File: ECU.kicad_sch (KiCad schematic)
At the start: 0 parts

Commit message: ECU
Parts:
- added K1: Relay_DPDT, symbol Relay:Relay_DPDT
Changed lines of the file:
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@@
 	(generator_version "9.0")
 	(paper "A4")
+	(symbol
+		(lib_id "Relay:Relay_DPDT")
+		(at 140.97 80.01 270)
+		(unit 1)
+		(exclude_from_sim no)
+		(in_bom yes)
+		(on_board yes)
+		(dnp no)
+		(fields_autoplaced yes)
+		(property "Reference" "K1"
+			(at 140.97 59.69 90)
+			(effects
+				(font
+					(size 1.27 1.27)
+				)
+			)
+		)
+		(property "Value" "Relay_DPDT"
+			(at 140.97 62.23 90)
+			(effects
+				(font
+					(size 1.27 1.27)
+				)
+			)
+		)
+		(property "Footprint" ""
+			(at 139.7 96.52 0)
+			(effects
+				(font
+					(size 1.27 1.27)
+				)
+				(justify left)
+				(hide yes)
+			)
+		)
+		(property "Datasheet" "~"
+			(at 140.97 80.01 0)
+			(effects
+				(font
+					(size 1.27 1.27)
+				)
+				(hide yes)
+			)
+		)
+		(property "Description" "Relay DPDT, monostable, EN50005"
+			(at 140.97 80.01 0)
+			(effects
+				(font
+					(size 1.27 1.27)
+				)
+				(hide yes)
+			)
+		)
+		(pin "11"
+		)
+		(pin "22"
+		)
+		(pin "A1"
+		)
+		(pin "A2"
+		)
+		(pin "12"
+		)
+		(pin "14"
+		)
+		(pin "24"
+		)
+		(pin "21"
+		)
+		(instances
+			(project ""
+				(path "/ae51d245-8015-483d-be59-5a0db9fda221"
+					(reference "K1")
+					(unit 1)
+				)
+			)
+		)
+	)
+	(sheet_instances
+		(path "/"
+			(page "1")
+		)
+	)
+	(embedded_fonts no)
 )

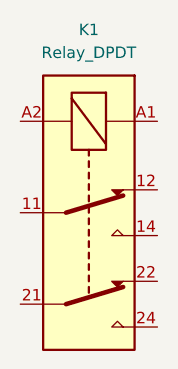
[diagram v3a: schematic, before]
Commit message: Connexion
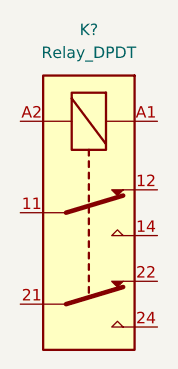
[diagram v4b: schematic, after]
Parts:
- renumbered K1 to K?
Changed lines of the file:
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@@
 		(dnp no)
 		(fields_autoplaced yes)
-		(property "Reference" "K1"
+		(property "Reference" "K?"
 			(at 140.97 59.69 90)
 			(effects
@@
 		)
 		(instances
+			(project "TEST"
+				(path "/6f31461c-1ce3-4669-a628-d5dc5fed8080/4e587e05-a25c-4fa2-aac4-623eb9b4720a"
+					(reference "K?")
+					(unit 1)
+				)
+			)
 			(project ""
 				(path "/ae51d245-8015-483d-be59-5a0db9fda221"
